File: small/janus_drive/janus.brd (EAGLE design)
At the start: 33 x 33.7 mm, 28 parts, among them IC1 LM741

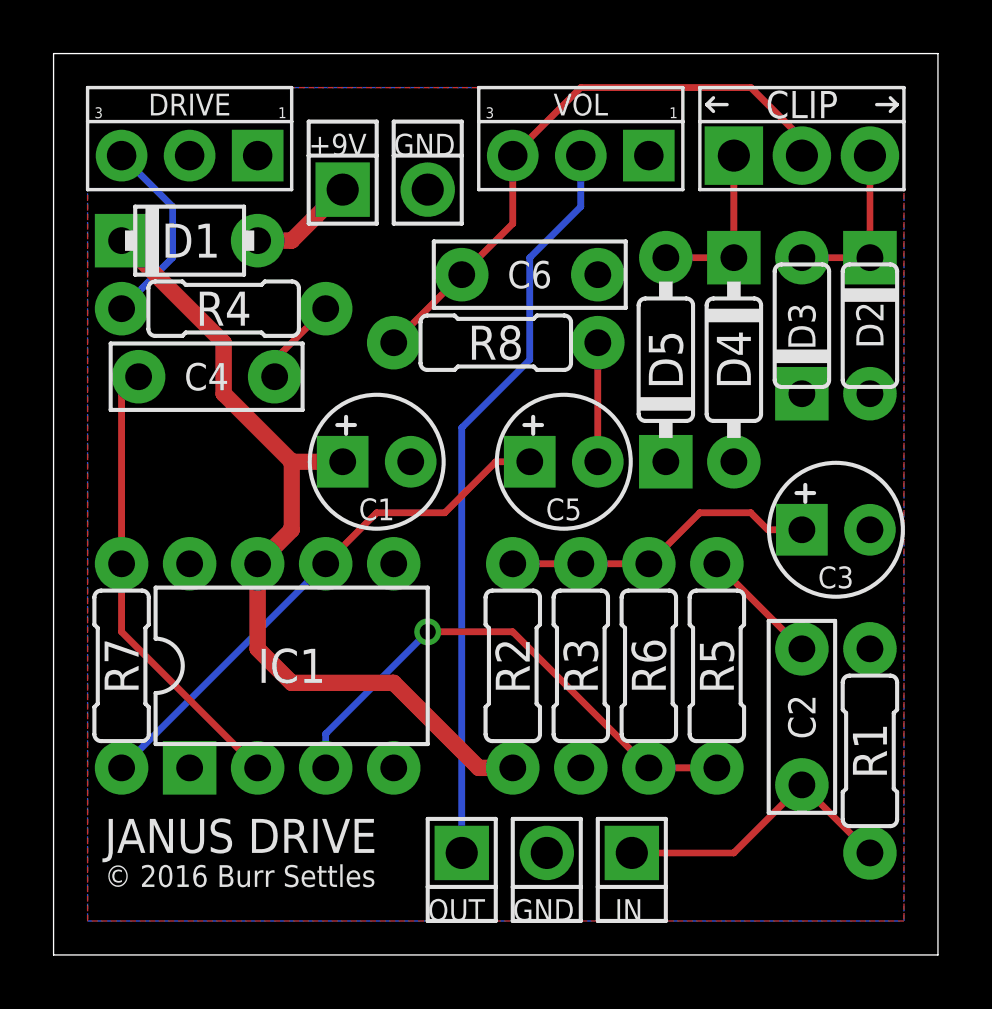
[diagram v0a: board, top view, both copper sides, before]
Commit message: updates to a few small pedals
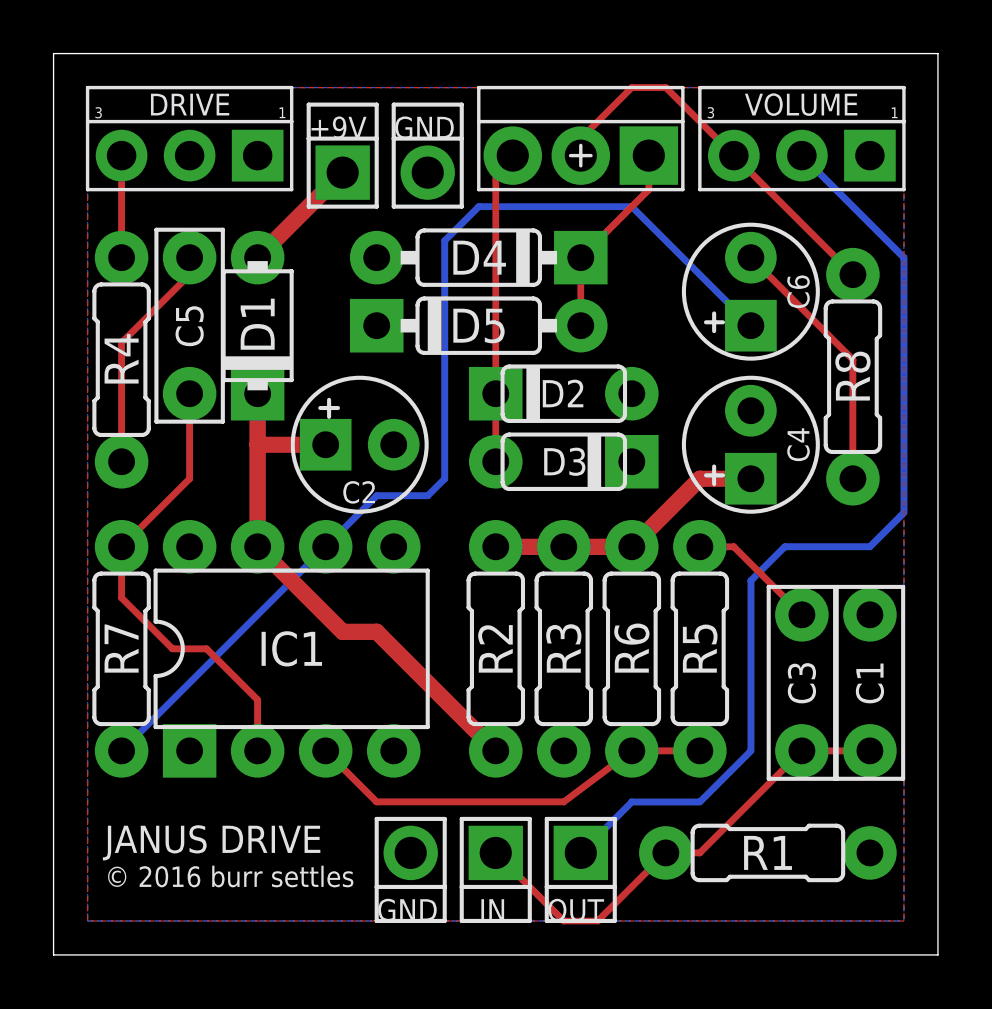
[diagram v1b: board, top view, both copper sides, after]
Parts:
- removed VOL: 100kA, potentiometers:PADS_SMALL
- added VOLUME: 100kA, potentiometers:PADS_SMALL
- C1: value 47u -> 2n2; device capacitors-elec:050_020_1 -> capacitors-film:BOX_SMALL
- C2: value 10n -> 47u; device capacitors-film:BOX_SMALL -> capacitors-elec:050_020_1
- C3: value 10u -> 10n; device capacitors-elec:050_020_1 -> capacitors-film:BOX_SMALL
- C4: value 47n -> 10u; device capacitors-film:BOX_SMALL -> capacitors-elec:050_020_1
- C5: value 4u7 -> 47n; device capacitors-elec:050_020_1 -> capacitors-film:BOX_SMALL
- C6: value 1n -> 4u7; device capacitors-film:BOX_SMALL -> capacitors-elec:050_020_1
- R1: value 2M2 -> 1M
- moved C4 20.5 mm to (26.0, 19.1), turned to 90 degrees
- moved C1 20.2 mm to (30.5, 10.2), turned to 270 degrees
- moved C2 19.4 mm to (11.4, 19.1), turned to 0 degrees
- moved C5 14.9 mm to (5.08, 23.5), turned to 90 degrees
- moved R8 13.4 mm to (29.8, 21.6), turned to 90 degrees
- moved D2 11.7 mm to (19.1, 21.0), turned to 0 degrees
- moved D4 10.3 mm to (15.9, 26.0), turned to 180 degrees
- moved D3 10.2 mm to (19.1, 18.4), turned to 180 degrees
- moved C6 8.28 mm to (26.0, 24.8), turned to 90 degrees
- moved CLIP 8.26 mm to (19.7, 29.8), flipped to the bottom
- moved D5 7.10 mm to (15.9, 23.5), turned to 0 degrees
- moved C3 5.85 mm to (27.9, 10.2), turned to 270 degrees
- moved R1 5.39 mm to (26.7, 3.81), turned to 180 degrees
- moved PAD2 5.08 mm to (16.5, 3.81)
- moved PAD3 5.08 mm to (13.3, 3.81)
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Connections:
- net CLIP: now also VOLUME.3; no longer C6.2, VOL.3
- net GND: now also C1.1, C2.-, C4.-, VOLUME.1; no longer C1.-, C3.-, C6.1, VOL.1
- net IN: now also C1.2, C3.2; no longer C2.2
- net N$1: now also C3.1; no longer C2.1
- net N$12: now also C2.+; no longer C1.+
- net N$3: now also C5.1; no longer C4.1
- net N$4: now also C5.2; no longer C4.2
- net N$5: now also C6.+; no longer C5.+
- net N$6: now also C6.-; no longer C5.-
- net N$8: now also C4.+; no longer C3.+
- net OUT: now also VOLUME.2; no longer VOL.2
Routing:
- net N$5: track 20.0 -> 39.0 mm
- net N$12: track 31.7 -> 20.3 mm
- net OUT: track 27.9 -> 36.0 mm
- net CLIP: track 22.1 -> 14.5 mm
- net IN: track 11.0 -> 17.7 mm
- net N$6: track 4.45 -> 9.83 mm
- net N$4: track 3.33 -> 8.67 mm
- net N$7: track 6.35 -> 11.7 mm
- net N$2: track 19.6 -> 15.4 mm, vias 1 -> 0
- net N$10: track 7.29 -> 3.81 mm
- net N$8: track 11.8 -> 10.6 mm
- net N$9: track 6.35 -> 7.40 mm
- net +9V: track 3.96 -> 4.49 mm
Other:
- board text added: "© 2016 burr settles"
- board text removed: "© 2016 Burr Settles"
